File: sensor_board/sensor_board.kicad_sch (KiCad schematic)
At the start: 4 parts, among them J1 Conn_01x04_Pin, U1 TSL25911FN

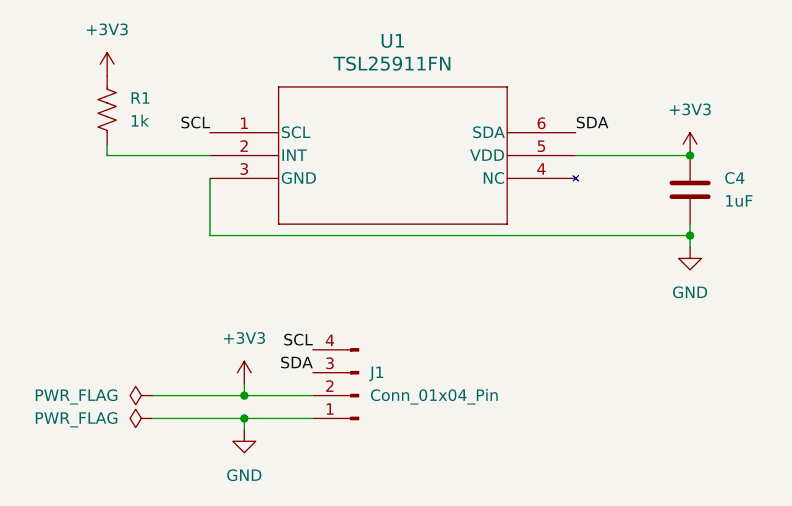
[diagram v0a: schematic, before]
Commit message: Fixed pins, minor changes, removed power isolation
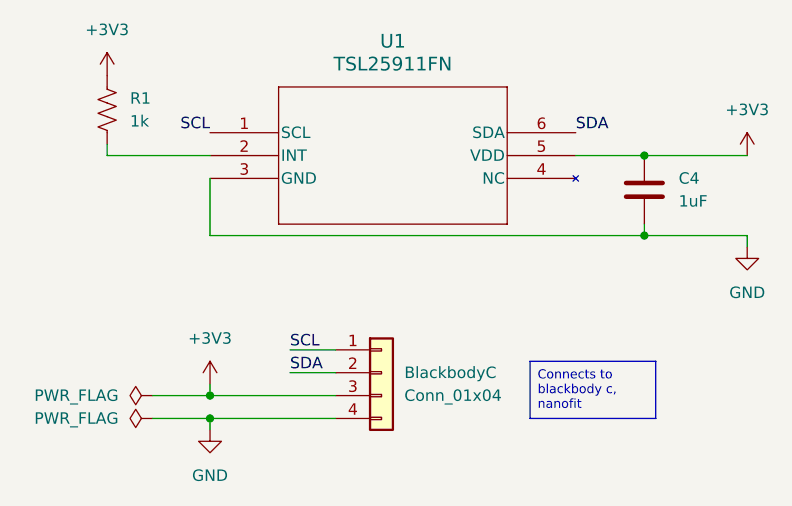
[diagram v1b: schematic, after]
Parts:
- removed J1: Conn_01x04_Pin, symbol Connector:Conn_01x04_Pin
- added BlackbodyC: Conn_01x04, symbol Connector_Generic:Conn_01x04
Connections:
- net +3V3: now also BlackbodyC.3 (Pin_3)
- net GND: now also BlackbodyC.4 (Pin_4)
- net SCL: now also BlackbodyC.1 (Pin_1)
- net SDA: now also BlackbodyC.2 (Pin_2)
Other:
- moved on the sheet: C4
